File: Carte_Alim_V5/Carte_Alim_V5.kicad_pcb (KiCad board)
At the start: 2 copper layers, 68 x 40.5 mm, 39 parts, among them J1 BAT_IN, J2 BAT_IN, U1 SIC466ED-T1-GE3

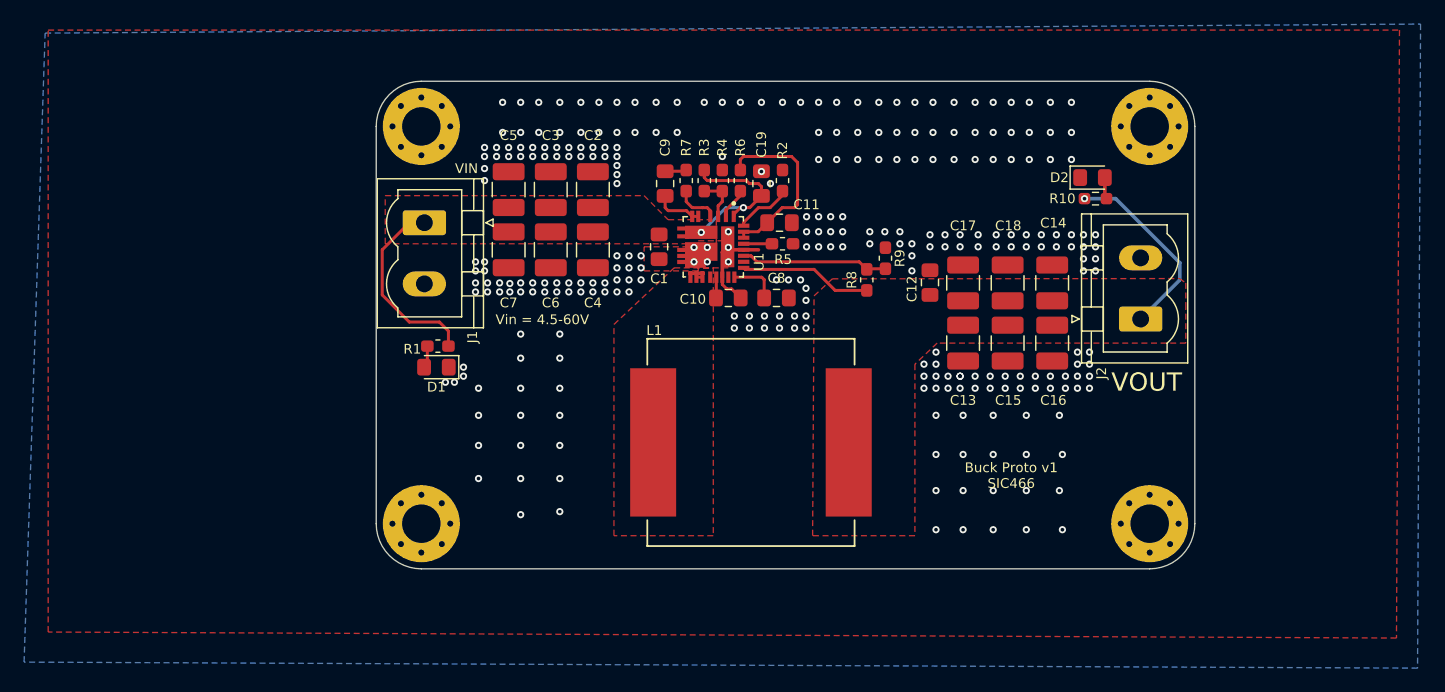
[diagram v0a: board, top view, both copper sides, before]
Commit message: lots of stuf
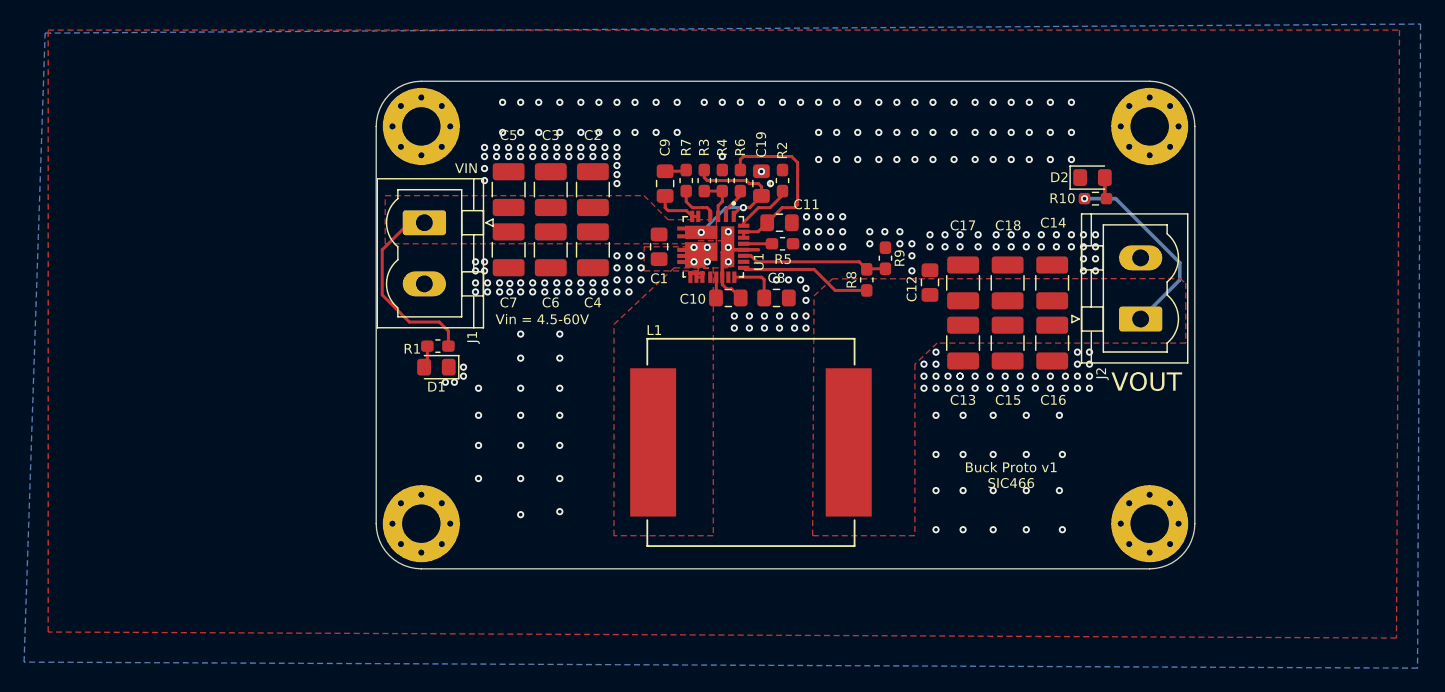
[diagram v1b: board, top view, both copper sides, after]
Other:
- net class Default removed
